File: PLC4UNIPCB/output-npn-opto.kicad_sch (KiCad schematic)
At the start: 3 parts

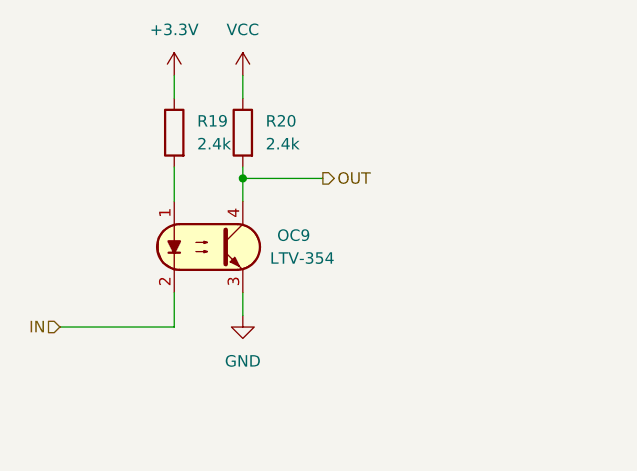
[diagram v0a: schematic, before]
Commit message: Add files via upload
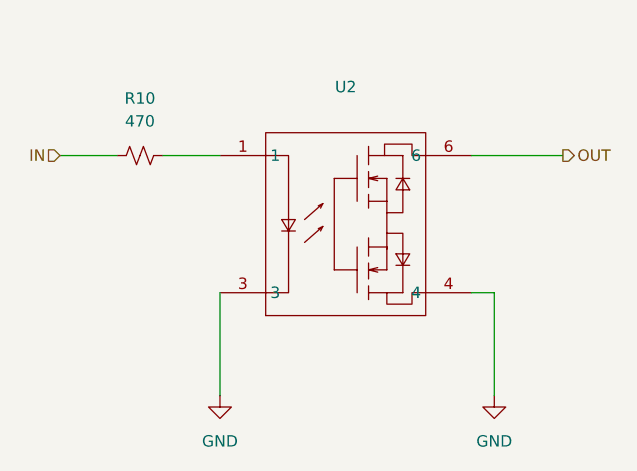
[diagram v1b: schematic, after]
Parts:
- removed OC9: FOD817S, Package_DIP_AKL:SMDIP-4_W9.53mm, symbol Optocoupler_AKL:FOD817S
- removed R19, R20: 2.4k, Resistor_SMD_AKL:R_0603_1608Metric, symbol Resistor_AKL:R_0603
- added R10: 470, PCM_SparkFun-Resistor:R_0603_1608Metric, symbol PCM_SparkFun-Resistor:4.7k_0603
- added U2: ~, EasyEDA_Lib:SOP-6_4P-L3.7-W4.6-P2.54-LS7.0-BL, symbol EasyEDA_Lib:TLP172AM(TPL,E
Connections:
- net GND: now also U2.3, U2.4
- net IN: now also R10.2
- net OUT: now also U2.6
- new net: R10.1, U2.1
